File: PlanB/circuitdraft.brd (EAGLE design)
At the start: 31.2 x 35.4 mm, 19 parts, among them Y1 CY16BPS

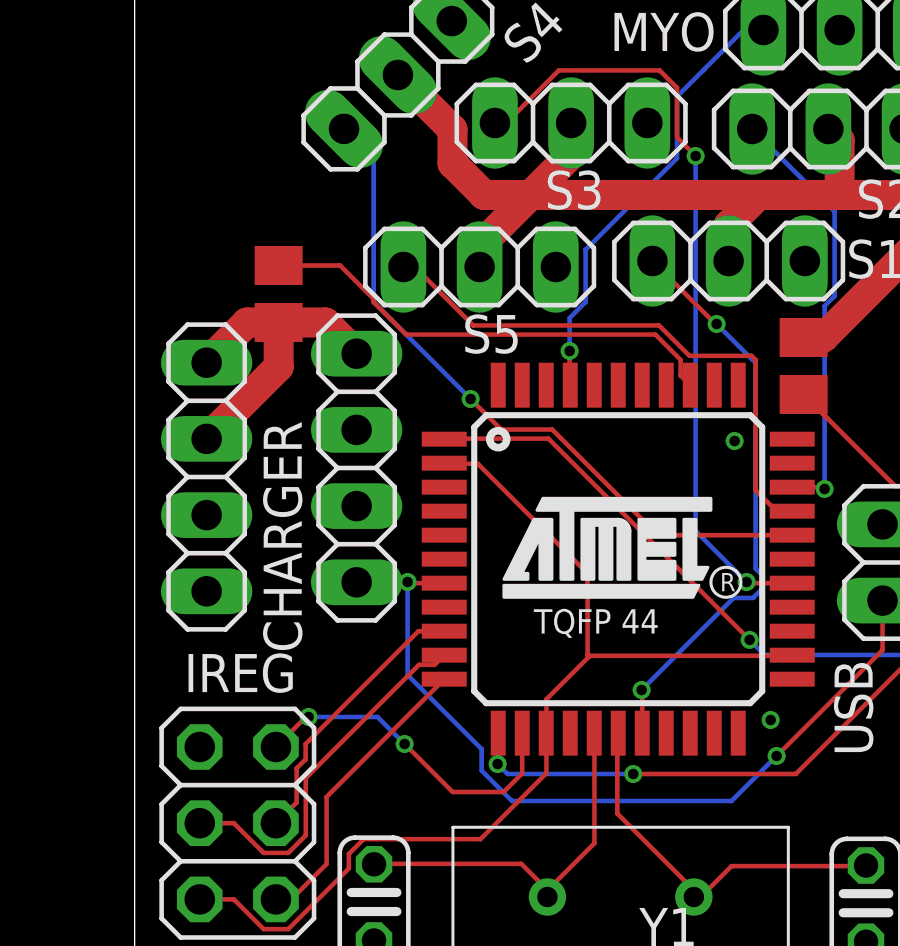
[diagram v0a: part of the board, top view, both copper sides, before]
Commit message: Error checking
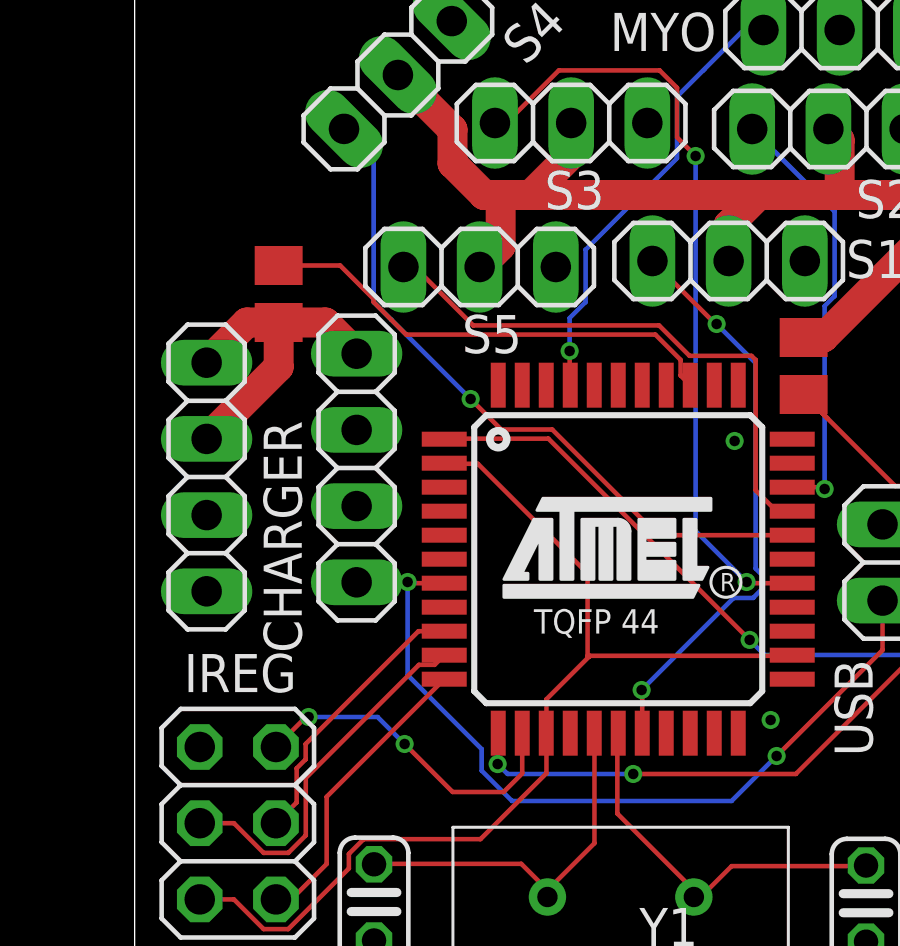
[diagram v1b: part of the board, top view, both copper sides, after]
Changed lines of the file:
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@@
 <contactref element="U$1" pad="7"/>
 <contactref element="CHARGER" pad="1"/>
-<wire x1="22.12" y1="17.66" x2="22.098" y2="17.6784" width="0.1524" layer="1"/>
 <via x="33.2" y="11.9" extent="1-16" drill="0.35"/>
 <wire x1="33.2" y1="11.9" x2="31.7" y2="10.4" width="0.1524" layer="16"/>
@@
 <wire x1="23.3694" y1="12.1306" x2="20.9" y2="14.6" width="0.1524" layer="16"/>
 <wire x1="20.9" y1="14.6" x2="20.9" y2="17.7" width="0.1524" layer="16"/>
-<wire x1="22.098" y1="17.6784" x2="21.9764" y2="17.8" width="0.1524" layer="1"/>
 <via x="20.9" y="17.7" extent="1-16" drill="0.35"/>
+<wire x1="33.2" y1="11.9" x2="36.73" y2="15.43" width="0.1524" layer="1"/>
+<wire x1="36.73" y1="15.43" x2="36.73" y2="17.08" width="0.1524" layer="1"/>
+<wire x1="19.2" y1="17.69" x2="20.89" y2="17.69" width="0.1524" layer="16"/>
+<wire x1="20.89" y1="17.69" x2="20.9" y2="17.7" width="0.1524" layer="16"/>
 <wire x1="22.12" y1="17.66" x2="20.94" y2="17.66" width="0.1524" layer="1"/>
 <wire x1="20.94" y1="17.66" x2="20.9" y2="17.7" width="0.1524" layer="1"/>
-<wire x1="19.2" y1="17.69" x2="19.21" y2="17.7" width="0.1524" layer="1"/>
-<wire x1="19.21" y1="17.7" x2="20.9" y2="17.7" width="0.1524" layer="1"/>
-<wire x1="33.2" y1="11.9" x2="36.73" y2="15.43" width="0.1524" layer="1"/>
-<wire x1="36.73" y1="15.43" x2="36.73" y2="17.08" width="0.1524" layer="1"/>
 </signal>
 <signal name="MISO">
@@
 <wire x1="24.2306" y1="11.3" x2="23.9" y2="11.6306" width="0.1524" layer="16"/>
 <via x="23.9" y="11.6306" extent="1-16" drill="0.35"/>
-<wire x1="23.9" y1="11.6306" x2="23.9" y2="12.64" width="0.1524" layer="1"/>
-<wire x1="23.9" y1="12.64" x2="23.92" y2="12.66" width="0.1524" layer="1"/>
+<wire x1="23.92" y1="12.66" x2="23.92" y2="11.6506" width="0.1524" layer="1"/>
+<wire x1="23.92" y1="11.6506" x2="23.9" y2="11.6306" width="0.1524" layer="1"/>
 </signal>
 <signal name="GND">
@@
 <via x="33" y="13.1" extent="1-16" drill="0.35"/>
 <contactref element="USB" pad="2"/>
-<wire x1="37.465" y1="32.8" x2="35.3" y2="36.1" width="0" layer="19" extent="1-1"/>
-<wire x1="40.8" y1="29.13" x2="37.465" y2="32.8" width="0" layer="19" extent="1-1"/>
-<wire x1="40.8" y1="26.59" x2="40.8" y2="29.13" width="0" layer="19" extent="1-1"/>
-<wire x1="40.9" y1="23.44" x2="40.8" y2="26.59" width="0" layer="19" extent="1-1"/>
-<wire x1="34.14" y1="28.4" x2="37.465" y2="32.8" width="0" layer="19" extent="1-1"/>
-<wire x1="31.12" y1="24.26" x2="34.14" y2="28.4" width="0" layer="19" extent="1-1"/>
-<wire x1="31.8" y1="22.4" x2="31.12" y2="24.26" width="0" layer="19" extent="1-1"/>
-<wire x1="36.73" y1="19.62" x2="40.9" y2="23.44" width="0" layer="19" extent="1-1"/>
-<wire x1="33.72" y1="14.46" x2="36.73" y2="19.62" width="0" layer="19" extent="1-1"/>
-<wire x1="33" y1="13.1" x2="33.72" y2="14.46" width="0" layer="19" extent="1-1"/>
-<wire x1="24.72" y1="24.26" x2="31.12" y2="24.26" width="0" layer="19" extent="1-1"/>
-<wire x1="25.84" y1="28.2" x2="24.72" y2="24.26" width="0" layer="19" extent="1-1"/>
-<wire x1="22.12" y1="19.26" x2="24.72" y2="24.26" width="0" layer="19" extent="1-1"/>
-<wire x1="19.2" y1="20.23" x2="22.12" y2="19.26" width="0" layer="19" extent="1-1"/>
-<wire x1="19.2" y1="22.77" x2="19.2" y2="20.23" width="0" layer="19" extent="1-1"/>
-<wire x1="14.2" y1="19.93" x2="19.2" y2="20.23" width="0" layer="19" extent="1-1"/>
-<wire x1="14.2" y1="17.39" x2="14.2" y2="19.93" width="0" layer="19" extent="1-1"/>
-<wire x1="13.97" y1="12.2" x2="14.2" y2="17.39" width="0" layer="19" extent="1-1"/>
-<wire x1="28.89" y1="33" x2="25.84" y2="28.2" width="0" layer="19" extent="1-1"/>
-<wire x1="26.32" y1="12.66" x2="33" y2="13.1" width="0" layer="19" extent="1-1"/>
-<wire x1="40.7" y1="12.73" x2="33.72" y2="14.46" width="0" layer="19" extent="1-1"/>
-<wire x1="22.37105" y1="36.39605" x2="28.89" y2="33" width="0" layer="19" extent="1-1"/>
-<wire x1="36.18" y1="5.71" x2="33" y2="13.1" width="0" layer="19" extent="1-1"/>
-<wire x1="19.78" y1="5.75" x2="13.97" y2="12.2" width="0" layer="19" extent="1-1"/>
 </signal>
 <signal name="INTERRUPT">
@@
 <wire x1="35.3" y1="32.425" x2="34.925" y2="32.8" width="1" layer="1"/>
 <wire x1="32.6" y1="30.6" x2="25" y2="30.6" width="1" layer="1"/>
-<wire x1="23.3" y1="28.9" x2="23.3" y2="28.2" width="1" layer="1"/>
-<wire x1="25" y1="30.6" x2="23.3" y2="28.9" width="1" layer="1"/>
 <wire x1="26.35" y1="33" x2="26.35" y2="31.95" width="1" layer="1"/>
 <wire x1="26.35" y1="31.95" x2="25" y2="30.6" width="1" layer="1"/>
@@
 <wire x1="22.3956" y1="32.7794" x2="22.3956" y2="31.65213125" width="1" layer="1"/>
 <wire x1="22.3956" y1="31.65213125" x2="23.44773125" y2="30.6" width="1" layer="1"/>
-<wire x1="23.44773125" y1="30.6" x2="25" y2="30.6" width="1" layer="1"/>
+<wire x1="23.44773125" y1="30.6" x2="24" y2="30.6" width="1" layer="1"/>
+<wire x1="24" y1="30.6" x2="25" y2="30.6" width="1" layer="1"/>
 <wire x1="40.8" y1="34.21" x2="40.8" y2="31.67" width="1" layer="1"/>
 <contactref element="MYO" pad="1"/>
@@
 <wire x1="34.75773125" y1="25.85" x2="34.1" y2="25.85" width="1" layer="1"/>
 <wire x1="39.45213125" y1="30.5444" x2="34.75773125" y2="25.85" width="1" layer="1"/>
+<wire x1="24" y1="30.6" x2="24" y2="28.9" width="1" layer="1"/>
+<wire x1="24" y1="28.9" x2="23.3" y2="28.2" width="1" layer="1"/>
 </signal>
 <signal name="N$9">
